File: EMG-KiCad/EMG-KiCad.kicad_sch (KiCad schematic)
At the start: 40 parts, among them J1 Conn_01x03_Socket, J2 Conn_01x03_Socket, U1 AD623, U2 OPA1662D, U3 OPA1662D, U4 OPA1662D, U5 OPA1662D, U6 OPA1662D, U7 LDO 3.3, U8 LDO 1.5, U9 OPA1662D

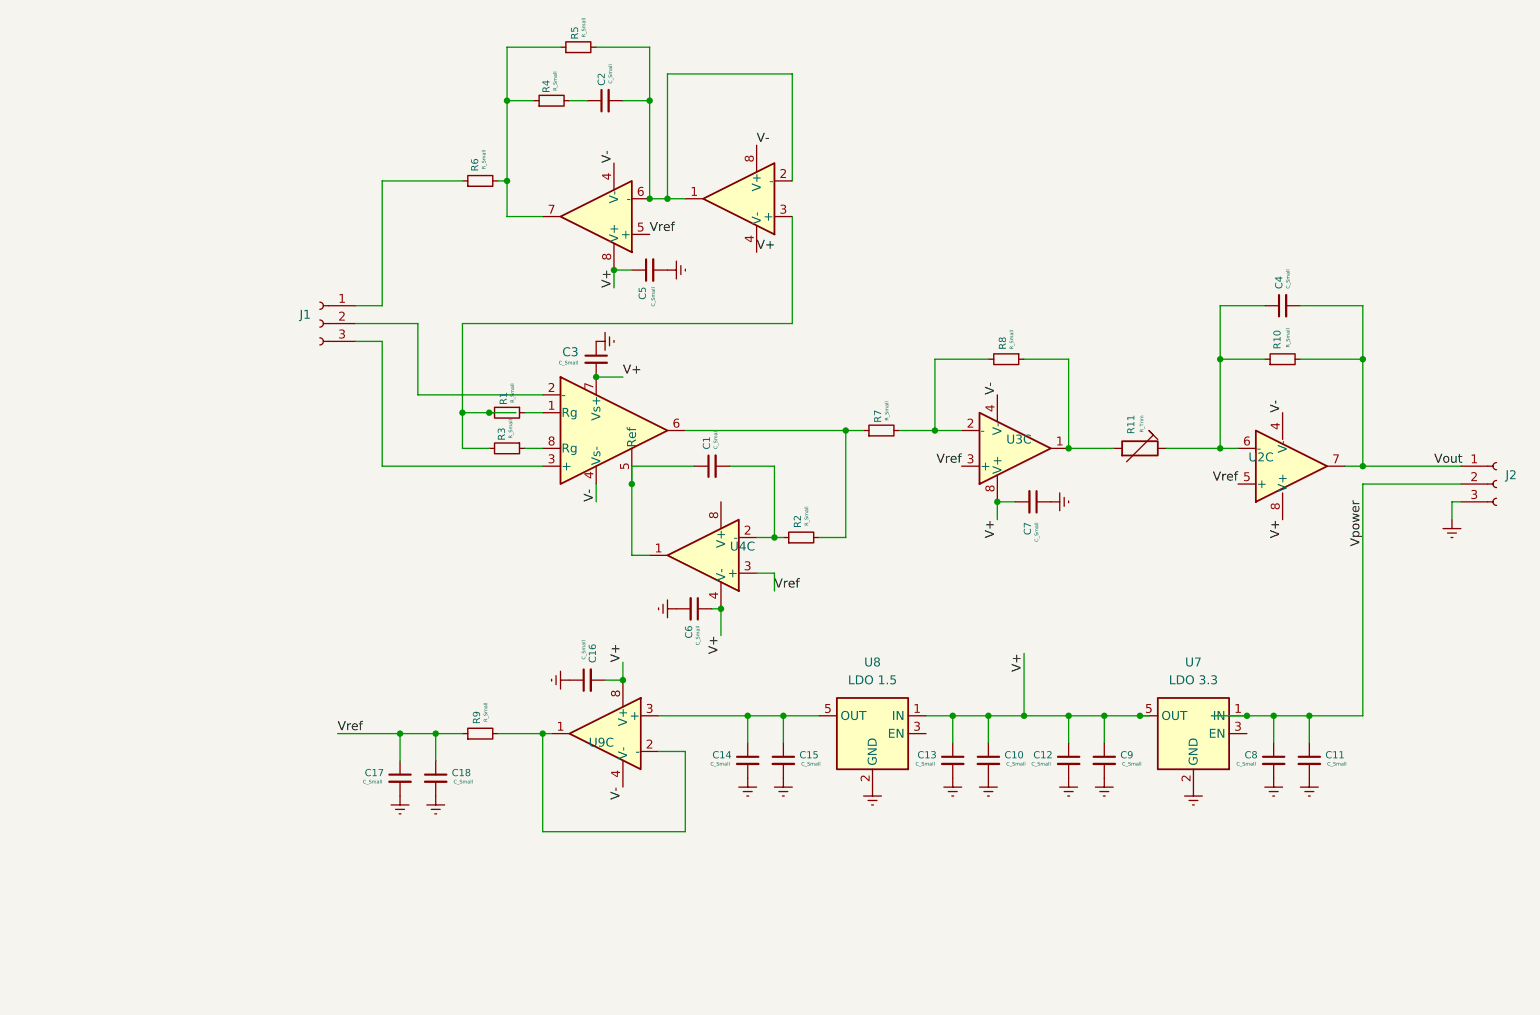
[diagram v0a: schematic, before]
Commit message: Complete schematic and add custom library
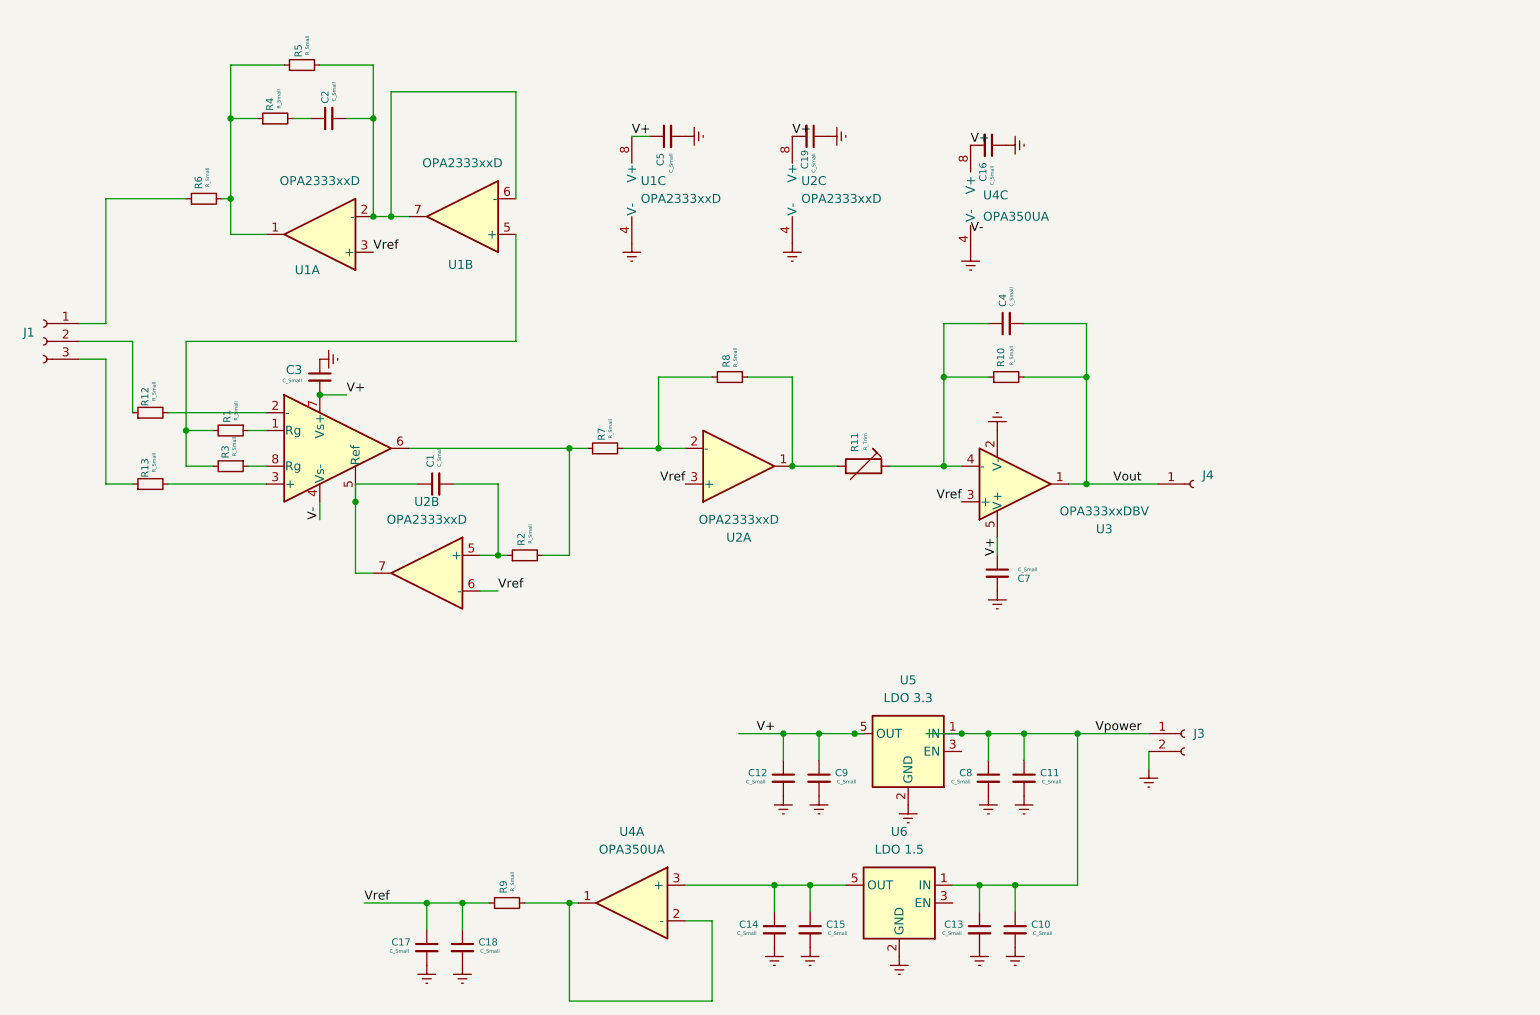
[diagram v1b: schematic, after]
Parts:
- removed C6: C_Small, symbol Device:C_Small
- removed J2: Conn_01x03_Socket, symbol Connector:Conn_01x03_Socket
- removed U2, U3, U4, U5, U6, U9: OPA1662D, Package_SO:SOIC-8_3.9x4.9mm_P1.27mm, symbol Amplifier_Operational:OPA1662D
- added C19: C_Small, Capacitor_SMD:C_0603_1608Metric_Pad1.08x0.95mm_HandSolder, symbol Device:C_Small
- added J3: Conn_01x02_Socket, Connector_Samtec_HPM_THT:Samtec_HPM-02-05-x-S_Straight_1x02_Pitch5.08mm, symbol Connector:Conn_01x02_Socket
- added J4: Conn_01x01_Socket, Connector_Samtec_HPM_THT:Samtec_HPM-01-05-x-S_Straight_1x01_Pitch5.08mm, symbol Connector:Conn_01x01_Socket
- added R12, R13: R_Small, Resistor_SMD:R_0603_1608Metric_Pad0.98x0.95mm_HandSolder, symbol Device:R_Small
- added U1, U2: OPA2333xxD, Package_SO:SOIC-8_3.9x4.9mm_P1.27mm, symbol Amplifier_Operational:OPA2333xxD
- added U3: OPA333xxDBV, Package_TO_SOT_SMD:SOT-23-5, symbol Amplifier_Operational:OPA333xxDBV
- added U4: OPA350UA, Package_SO:SOIC-8_5.3x6.2mm_P1.27mm, symbol LIMB_EMG_Library:OPA350UA
- C1, C10, C11, C12, C13, C14, C15, C16, C17, C18, C2, C3, C4, C5, C7, C8, C9: footprint (none) -> Capacitor_SMD:C_0603_1608Metric_Pad1.08x0.95mm_HandSolder
- J1: footprint (none) -> Connector_Samtec_HPM_THT:Samtec_HPM-03-05-x-S_Straight_1x03_Pitch5.08mm
- R1, R10, R11, R2, R3, R4, R5, R6, R7, R8, R9: footprint (none) -> Resistor_SMD:R_0603_1608Metric_Pad0.98x0.95mm_HandSolder
- U0: renamed from U1; footprint (none) -> Package_SO:SOIC-8_5.3x6.2mm_P1.27mm
- renumbered U7 to U5, U8 to U6
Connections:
- net Earth: now also C7.2, C19.1, J3.2 (Pin_2), U1.4 (V-), U2.4 (V-), U3.2 (V-), U4.4 (V-); no longer C7.1
- net V+: now also C7.1, C19.2, U1.8 (V+), U2.8 (V+), U3.5 (V+), U4.8 (V+); no longer C10.1, C13.1, C7.2, U6.1 (IN)
- net Vout: now also J4.1 (Pin_1), U3.1
- net Vpower: now also C10.1, C13.1, U6.1 (IN), J3.1 (Pin_1)
- net Vref: now also U1.3 (+), U2.3 (+), U2.6 (-), U3.3 (+)
- net at C1.1, U0.5 (Ref): now also U2.7
- net at C1.2, R2.1: now also U2.5 (+)
- net at R4.1, R5.1, R6.2: now also U1.1
- net at C2.2, R5.2: now also U1.2 (-), U1.6 (-), U1.7
- net at C14.1, C15.1, U6.5 (OUT): now also U4.3 (+)
- net at R7.2, R8.2: now also U2.2 (-)
- net at R11.2, R8.1: now also U2.1
- net at C4.1, R10.1, R11.1: now also U3.4 (-)
- net at R9.2: now also U4.1, U4.2 (-)
- net at U0.2 (-): now also R12.2; no longer J1.2 (Pin_2)
- net at J1.3 (Pin_3): now also R13.1; no longer U0.3 (+)
- net at R1.2, R3.2: now also U1.5 (+)
- new net: R13.2, U0.3 (+)
- new net: J1.2 (Pin_2), R12.1
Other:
- moved on the sheet: C1, C10, C11, C12, C13, C14, C15, C16, C17, C18, C2, C3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
